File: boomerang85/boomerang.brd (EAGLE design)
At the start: 99.2 x 91.7 mm, 16 parts

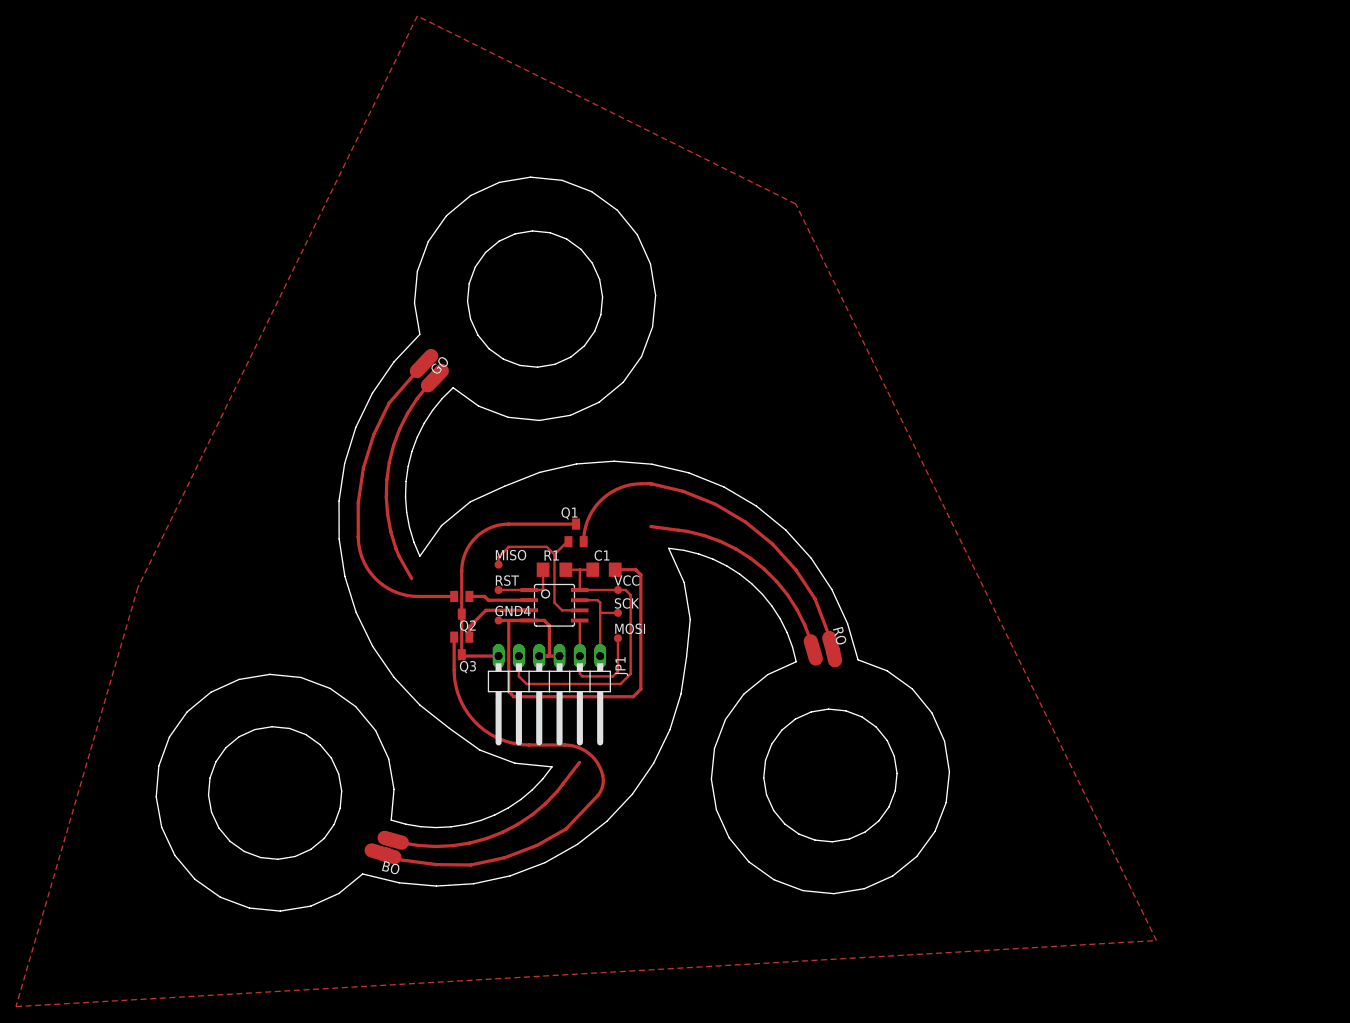
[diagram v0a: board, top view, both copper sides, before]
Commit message: moar awesome
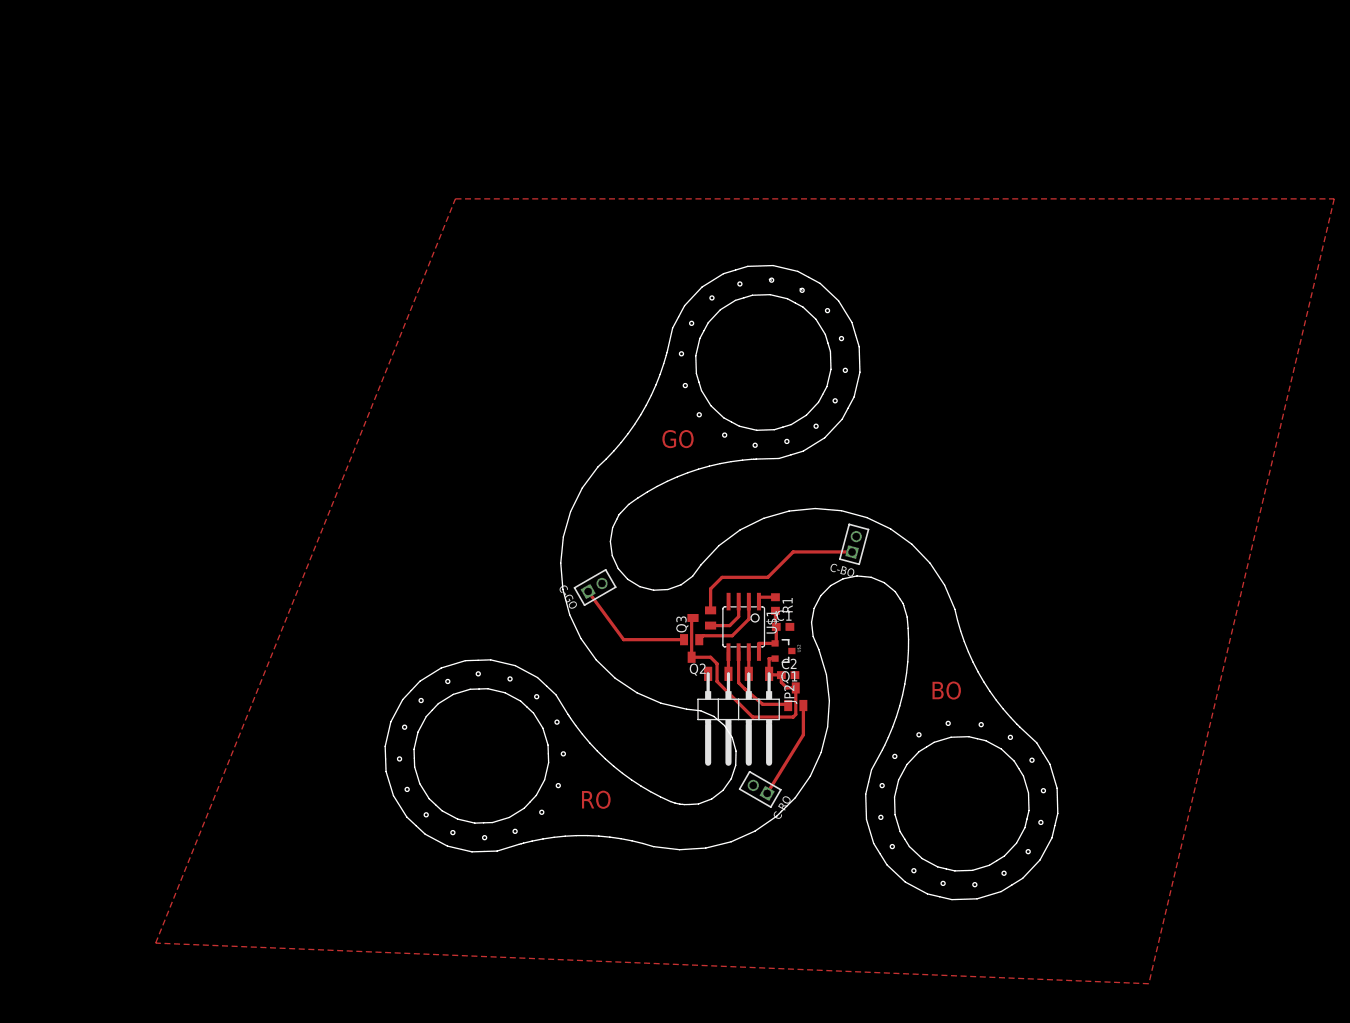
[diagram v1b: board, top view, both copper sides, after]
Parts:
- removed BO, GO, RO: (no value), wirepad:SMD1,27-2,54
- removed GND4, MISO, MOSI, RST, SCK, VCC: PTR1TP10R, testpad:TP10R
- removed JP1: (no value), pinhead:1X06/90
- added C-BO, C-GO, C-RO: (no value), pinhead:1X02M
- added C2: 100nF, resistor:C0603
- added JP2: (no value), pinhead-1:1X04SMD/90
- added U$2: LM3480IM4, SparkFun-PowerIC:SOT23-3
- C1: device resistor:C1206 -> resistor:C0603
- R1: device resistor:R1206 -> resistor:R0603
- moved Q1 34.3 mm to (10.5, -6.35)
- moved Q3 30.2 mm to (-1.27, 3.49), turned to 90 degrees
- moved Q2 29.2 mm to (-2.54, -0.32)
- moved R1 28.0 mm to (7.94, 5.24), turned to 270 degrees
- moved U$1 23.8 mm to (3.97, 2.38), turned to 180 degrees
- moved C1 23.5 mm to (8.89, 2.38)
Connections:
- removed net 3VD: JP1.6, Q1.3, Q2.3, Q3.3
- removed net VCC3: C1.1, JP1.5, R1.2, U$1.8, VCC.TP
- new net VCC: C2.1, JP2.1, Q1.3, Q2.3, Q3.3, U$2.2
- new net VCC_GOOD: C1.1, R1.2, U$1.8, U$2.1
- net BO: now also C-BO.1; no longer BO.1
- net GND: now also C-BO.2, C-GO.2, C-RO.2, C2.2, JP2.4, U$2.3; no longer GND4.TP, JP1.3, JP1.4
- net GO: now also C-GO.1; no longer GO.1
- net R: no longer MISO.TP
- net RES: no longer RST.TP
- net RO: now also C-RO.1; no longer RO.1
- net SCL: now also JP2.2; no longer JP1.1, SCK.TP
- net SDA: now also JP2.3; no longer JP1.2, MOSI.TP
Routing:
- net GND: track 146.0 -> 0.00 mm
- net BO: track 62.6 -> 22.3 mm
- net VCC3: track 39.8 -> 0.00 mm
- net RO: track 46.1 -> 12.3 mm
- net VCC: track 0.00 -> 33.0 mm
- net 3VD: track 31.9 -> 0.00 mm
- net GO: track 46.4 -> 15.0 mm
- net SDA: track 16.0 -> 2.72 mm
- net R: track 20.9 -> 11.1 mm
- net SCL: track 11.6 -> 2.72 mm
- net VCC_GOOD: track 0.00 -> 7.43 mm
- net RES: track 8.01 -> 2.62 mm
- net B: track 9.62 -> 5.86 mm
- net G: track 7.68 -> 9.46 mm
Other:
- board size 99.2 x 91.7 mm -> 84.1 x 79.3 mm
- board text added: "BO"
- board text added: "GO"
- board text added: "RO"

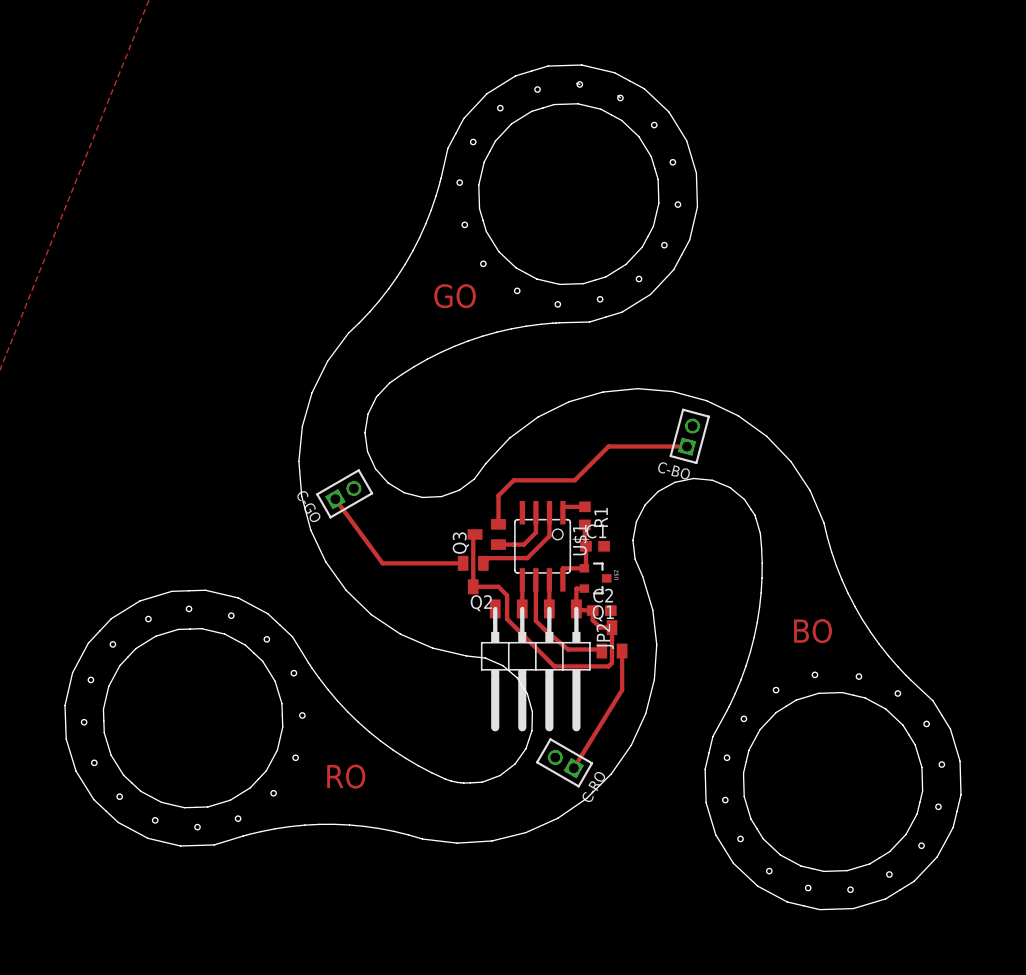
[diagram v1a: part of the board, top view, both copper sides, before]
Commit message: foo
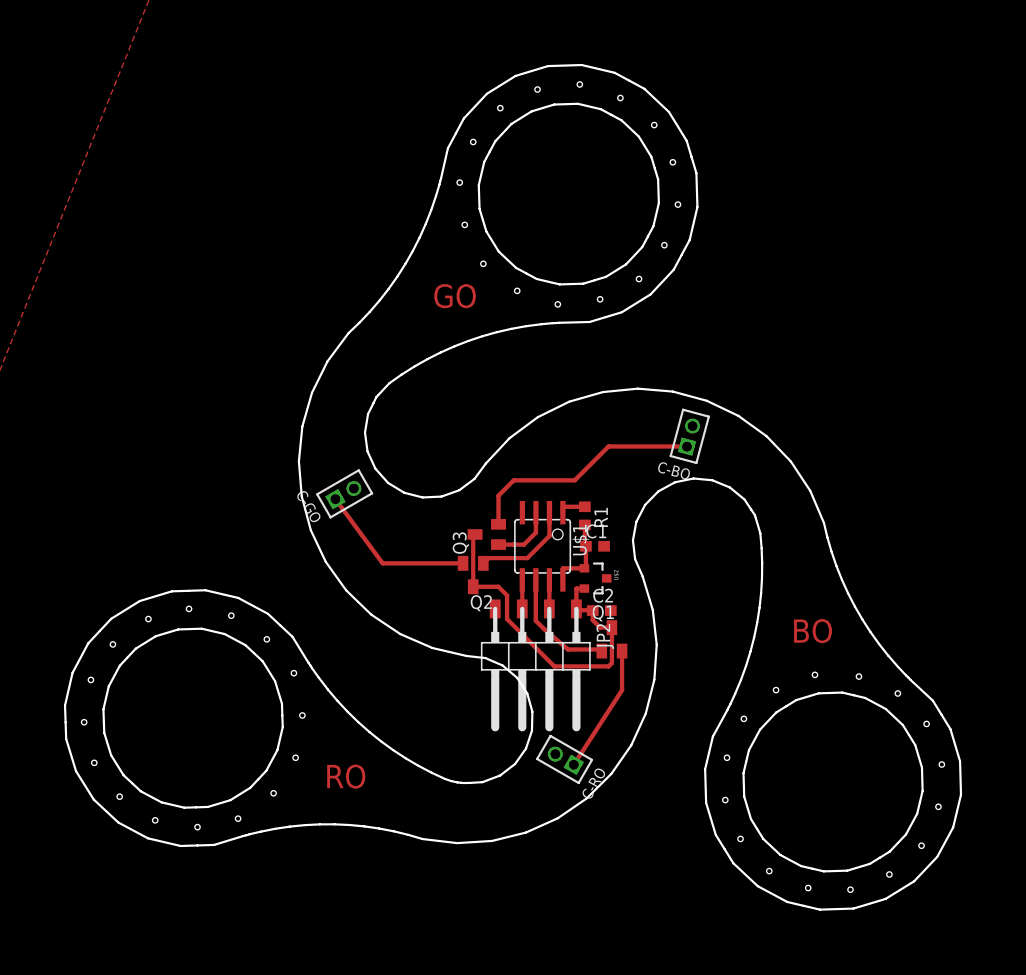
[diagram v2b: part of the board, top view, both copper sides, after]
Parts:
- moved C-RO 0.32 mm to (6.03, -17.6)
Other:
- outline, holes or cut-outs redrawn
